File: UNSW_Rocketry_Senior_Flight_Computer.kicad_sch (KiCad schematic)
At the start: 17 parts, among them U1 STM32L452RETx, Y1 8MHz

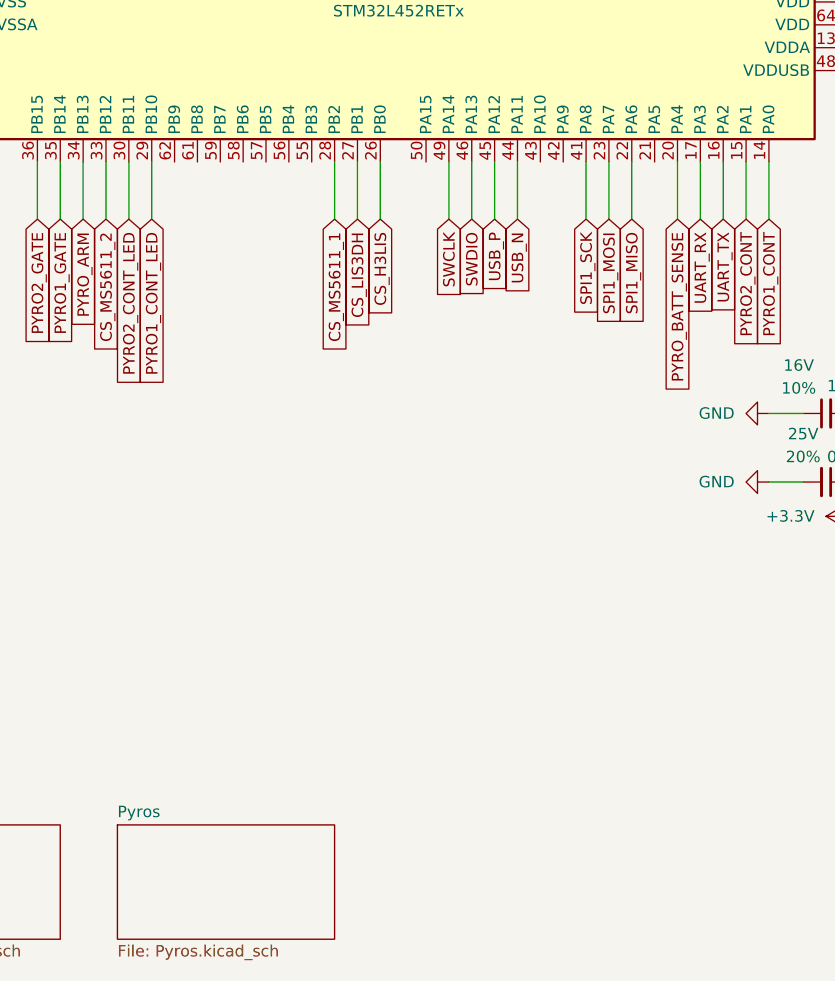
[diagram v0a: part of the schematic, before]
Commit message: feat: finish board (draft)
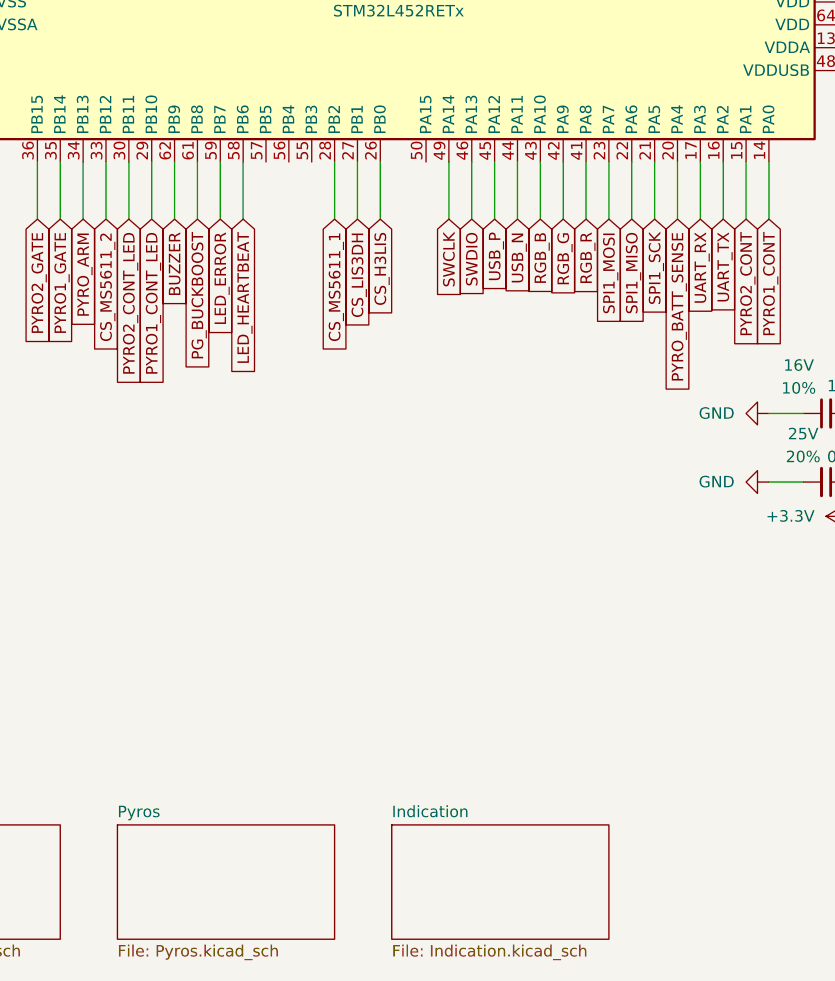
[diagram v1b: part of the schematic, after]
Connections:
- net SPI1_SCK: now also U1.21 (PA5); no longer U1.41 (PA8)
- net RGB_G: now reaches U1.42 (PA9)
- net RGB_B: now reaches U1.43 (PA10)
- net LED_HEARTBEAT: now reaches U1.58 (PB6)
- net LED_ERROR: now reaches U1.59 (PB7)
- net PG_BUCKBOOST: now reaches U1.61 (PB8)
- net BUZZER: now reaches U1.62 (PB9)
- new net RGB_R: U1.41 (PA8)
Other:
- added sheet Indication (Indication.kicad_sch)
